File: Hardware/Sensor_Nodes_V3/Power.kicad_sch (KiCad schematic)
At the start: 14 parts, among them U2 TPS563200, U4 AMS1117-3.3

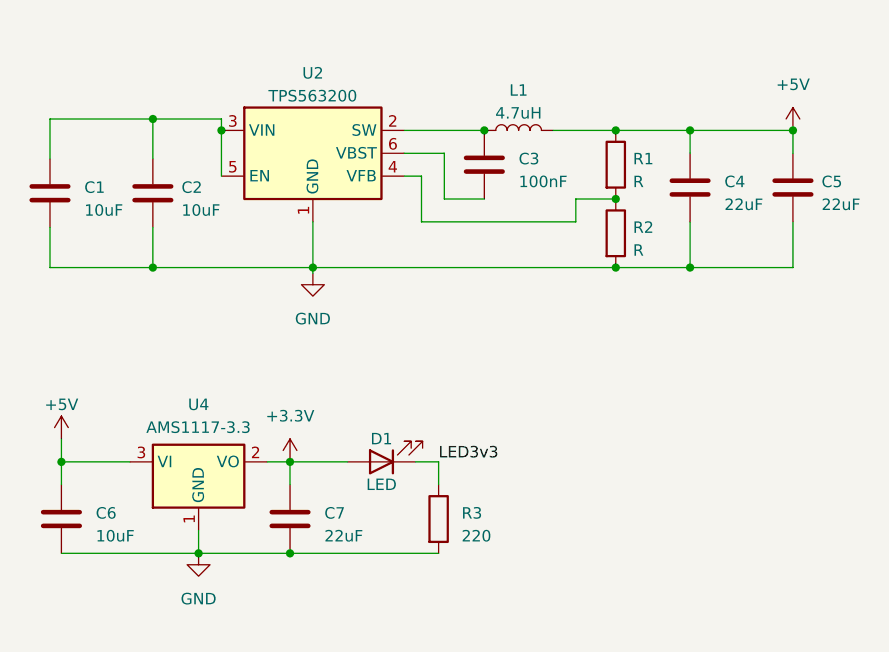
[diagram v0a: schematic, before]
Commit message: a lot of progress on V3, still need to test if bootloader works
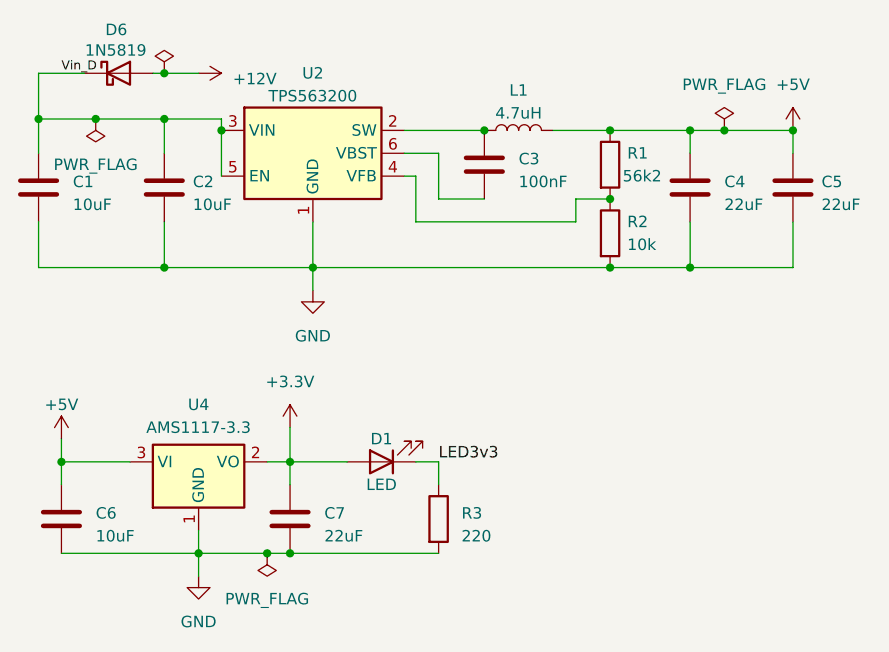
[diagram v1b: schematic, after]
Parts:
- added D6: 1N5819, Diode_SMD:D_SOD-323_HandSoldering, symbol Device:D_Schottky
- C1, C2: footprint (none) -> Capacitor_SMD:C_1206_3216Metric
- C3, C4, C5: footprint (none) -> Capacitor_SMD:C_0402_1005Metric
- C6: footprint Capacitor_SMD:C_0603_1608Metric -> Capacitor_SMD:C_0805_2012Metric
- L1: footprint (none) -> Inductor_SMD:L_Cenker_CKCS6045
- R1: value R -> 56k2; footprint (none) -> Resistor_SMD:R_0402_1005Metric
- R2: value R -> 10k; footprint (none) -> Resistor_SMD:R_0402_1005Metric
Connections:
- net Vin_D: now reaches C1.1, C2.1, U2.3 (VIN), U2.5 (EN)
- net Vin_D: now also D6.1 (K)
- new net +12V: D6.2 (A)
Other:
- moved on the sheet: C1, C2, R1, R2

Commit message: sync update
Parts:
- C1, C2: footprint Capacitor_SMD:C_1206_3216Metric -> Capacitor_SMD:C_0603_1608Metric
- C3: footprint Capacitor_SMD:C_0402_1005Metric -> Capacitor_SMD:C_0603_1608Metric
- C4, C5: footprint Capacitor_SMD:C_0402_1005Metric -> Resistor_SMD:R_0805_2012Metric
- C6: footprint Capacitor_SMD:C_0805_2012Metric -> Capacitor_SMD:C_0603_1608Metric
- R3: footprint Resistor_SMD:R_0603_1608Metric -> Resistor_SMD:R_0402_1005Metric
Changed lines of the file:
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@@
 			)
 		)
-		(property "Footprint" "Capacitor_SMD:C_1206_3216Metric"
+		(property "Footprint" "Capacitor_SMD:C_0603_1608Metric"
 			(at 22.5552 34.29 0)
 			(effects
@@
 			)
 		)
-		(property "Footprint" "Capacitor_SMD:C_0402_1005Metric"
+		(property "Footprint" "Resistor_SMD:R_0805_2012Metric"
 			(at 106.3752 34.29 0)
 			(effects
@@
 			)
 		)
-		(property "Footprint" "Capacitor_SMD:C_0402_1005Metric"
+		(property "Footprint" "Capacitor_SMD:C_0603_1608Metric"
 			(at 72.0852 31.75 0)
 			(effects
@@
 			)
 		)
-		(property "Footprint" "Capacitor_SMD:C_0805_2012Metric"
+		(property "Footprint" "Capacitor_SMD:C_0603_1608Metric"
 			(at 25.0952 71.12 0)
 			(effects
@@
 			)
 		)
-		(property "Footprint" "Resistor_SMD:R_0603_1608Metric"
+		(property "Footprint" "Resistor_SMD:R_0402_1005Metric"
 			(at 64.262 67.31 90)
 			(effects
@@
 			)
 		)
-		(property "Footprint" "Capacitor_SMD:C_0402_1005Metric"
+		(property "Footprint" "Resistor_SMD:R_0805_2012Metric"
 			(at 94.9452 34.29 0)
 			(effects
@@
 			)
 		)
-		(property "Footprint" "Capacitor_SMD:C_1206_3216Metric"
+		(property "Footprint" "Capacitor_SMD:C_0603_1608Metric"
 			(at 36.5252 34.29 0)
 			(effects
